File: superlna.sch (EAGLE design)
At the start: 7 parts, among them X1 SMA-142-0701-801/806, X2 SMA-142-0701-801/806

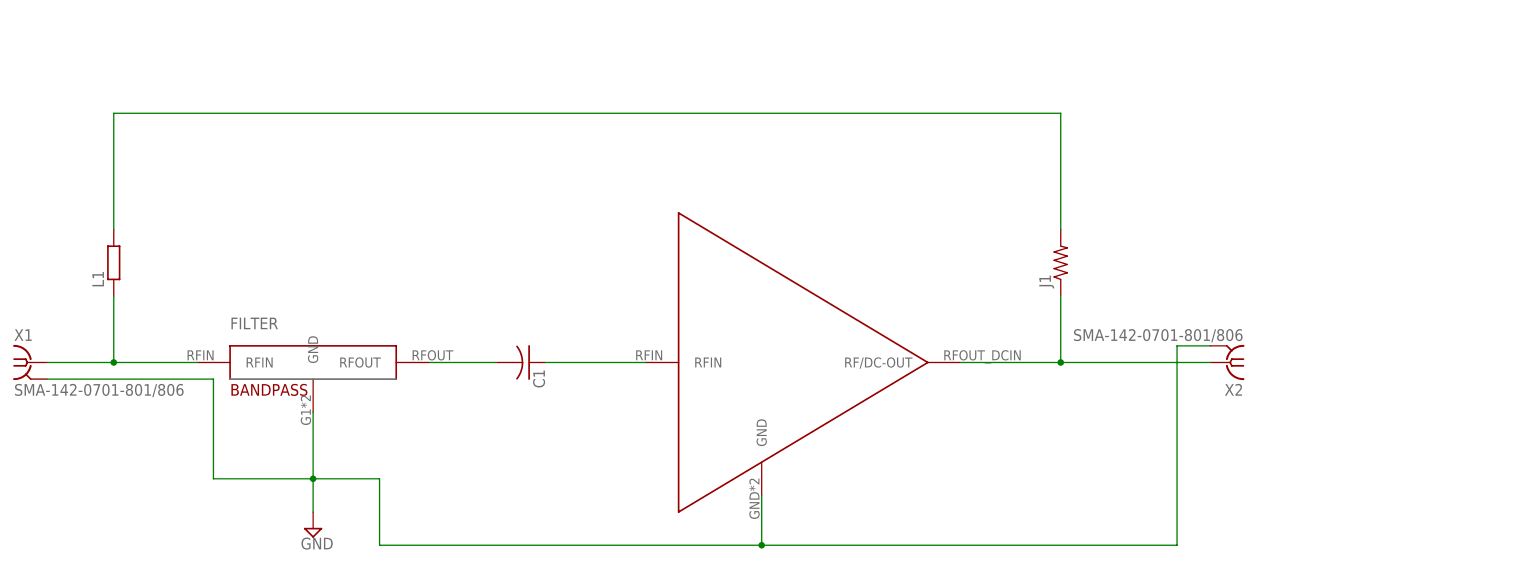
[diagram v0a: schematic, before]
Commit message: V1.0
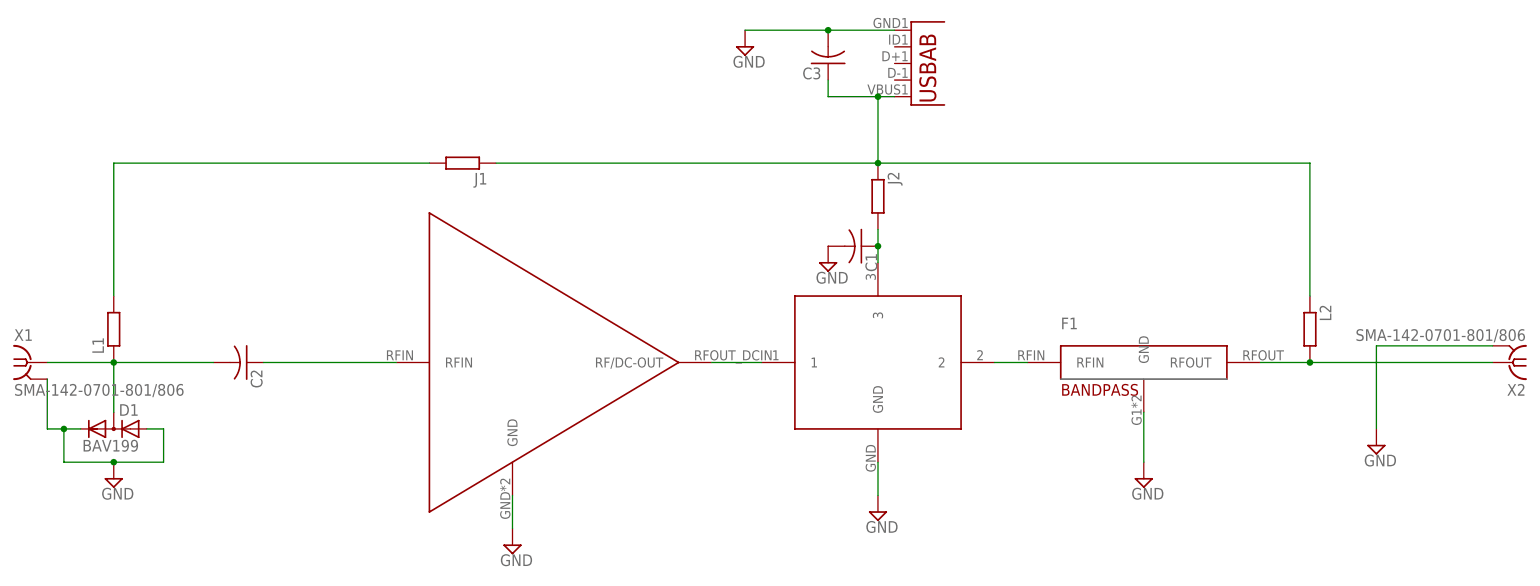
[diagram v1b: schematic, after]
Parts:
- removed FILTER: BANDPASS, custom:BANDPASS
- removed PSA4-5043+: AMP, custom:AMP
- added C2, C3: (no value), rcl:C-USC0402
- added D1: BAV199, diode:BAV199
- added F1: BANDPASS, custom:BANDPASS
- added J2, L2: (no value), rcl:R-EU_R0805
- added POWER: (no value), microusb:USB""
- added U1: BIASTEE, minicircuits:BIASTEE
- added U2: AMP, custom:AMP
- J1: device rcl:R-US_R0805 -> rcl:R-EU_R0805
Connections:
- removed net N$1: FILTER.RFIN, L1.1, X1.1
- removed net N$3: C1.2, FILTER.RFOUT
- new net BIASPOWER: C1.1, J2.2, U1.3
- new net N$4: C3.1, J1.1, J2.1, L2.1, POWER.VBUS
- new net N$6: F1.RFIN, U1.2
- new net RFIN: C2.2, D1.AC, L1.1, X1.1
- new net RFOUT: F1.RFOUT, L2.2, X2.1
- net GND: now also C1.2, C3.2, D1.A, D1.C, F1.GND, POWER.GND, U1.GND, U2.GND; no longer FILTER.GND, PSA4-5043+.GND
- net N$2: now also C2.1, U2.RFIN; no longer C1.1, PSA4-5043+.RFIN
- net N$5: now also U1.1, U2.RF/DC-OUT; no longer J1.1, PSA4-5043+.RF/DC-OUT, X2.1
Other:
- moved on the sheet: C1, L1, X2

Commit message: changes to V1
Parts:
- removed U2: AMP, custom:AMP
- added U$1: AMP, minicircuits:AMP
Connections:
- net GND: now also U$1.GND; no longer U2.GND
- net N$2: now also U$1.RFIN; no longer U2.RFIN
- net N$5: now also U$1.RF/DC-OUT; no longer U2.RF/DC-OUT
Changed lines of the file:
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@@
 <part name="SUPPLY5" library="supply2" deviceset="GND" device=""/>
 <part name="C2" library="rcl" deviceset="C-US" device="C0402"/>
-<part name="U2" library="custom" deviceset="AMP" device=""/>
 <part name="U1" library="minicircuits" deviceset="BIASTEE" device=""/>
 <part name="SUPPLY7" library="supply2" deviceset="GND" device=""/>
+<part name="U$1" library="minicircuits" deviceset="AMP" device=""/>
 </parts>
 <sheets>
@@
 <instance part="SUPPLY5" gate="GND" x="53.34" y="50.8"/>
 <instance part="C2" gate="G$1" x="-22.86" y="2.54" rot="R270"/>
-<instance part="U2" gate="G$1" x="17.78" y="2.54"/>
 <instance part="U1" gate="G$1" x="73.66" y="2.54"/>
 <instance part="SUPPLY7" gate="GND" x="73.66" y="-20.32"/>
+<instance part="U$1" gate="G$1" x="17.78" y="2.54"/>
 </instances>
 <busses>
@@
 <wire x1="17.78" y1="-17.78" x2="17.78" y2="-22.86" width="0.1524" layer="91"/>
 <pinref part="SUPPLY3" gate="GND" pin="GND"/>
-<pinref part="U2" gate="G$1" pin="GND"/>
+<pinref part="U$1" gate="G$1" pin="GND"/>
 </segment>
 <segment>
@@
 <segment>
 <wire x1="55.88" y1="2.54" x2="48.26" y2="2.54" width="0.1524" layer="91"/>
-<pinref part="U2" gate="G$1" pin="RF/DC-OUT"/>
 <pinref part="U1" gate="G$1" pin="1"/>
+<pinref part="U$1" gate="G$1" pin="RF/DC-OUT"/>
 </segment>
 </net>
@@
 <segment>
 <pinref part="C2" gate="G$1" pin="1"/>
-<pinref part="U2" gate="G$1" pin="RFIN"/>
+<pinref part="U$1" gate="G$1" pin="RFIN"/>
 <wire x1="-20.32" y1="2.54" x2="0" y2="2.54" width="0.1524" layer="91"/>
 </segment>
